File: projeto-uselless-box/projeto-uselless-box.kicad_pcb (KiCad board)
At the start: 2 copper layers, 128 x 94 mm, 13 parts, among them J2 Conn_Para_Fita, J3 Conn_Para_PowerBank, M1 Motor_Servo-Edit, M2 Motor_Servo-Edit, M3 Motor_Servo-Edit, Q1 TIP41, SW1 SW_DPST_x2

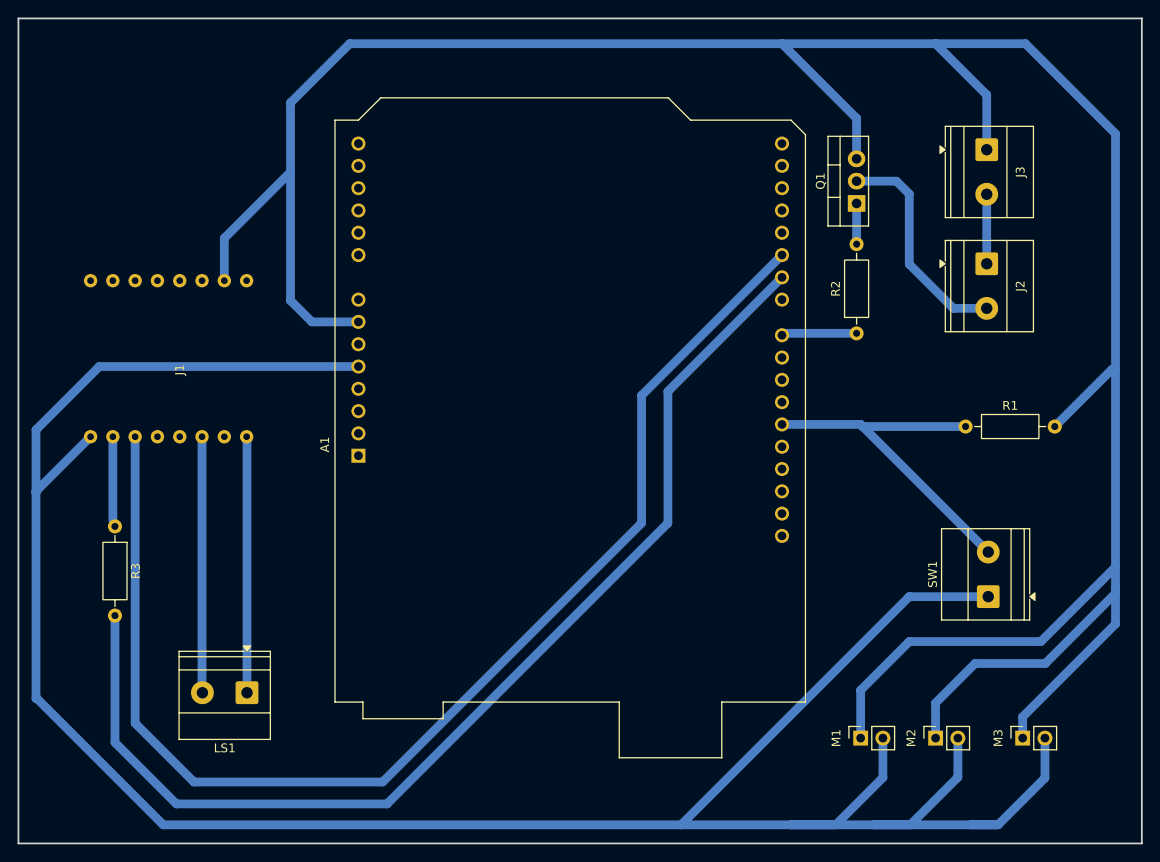
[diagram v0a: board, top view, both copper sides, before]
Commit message: Shorted
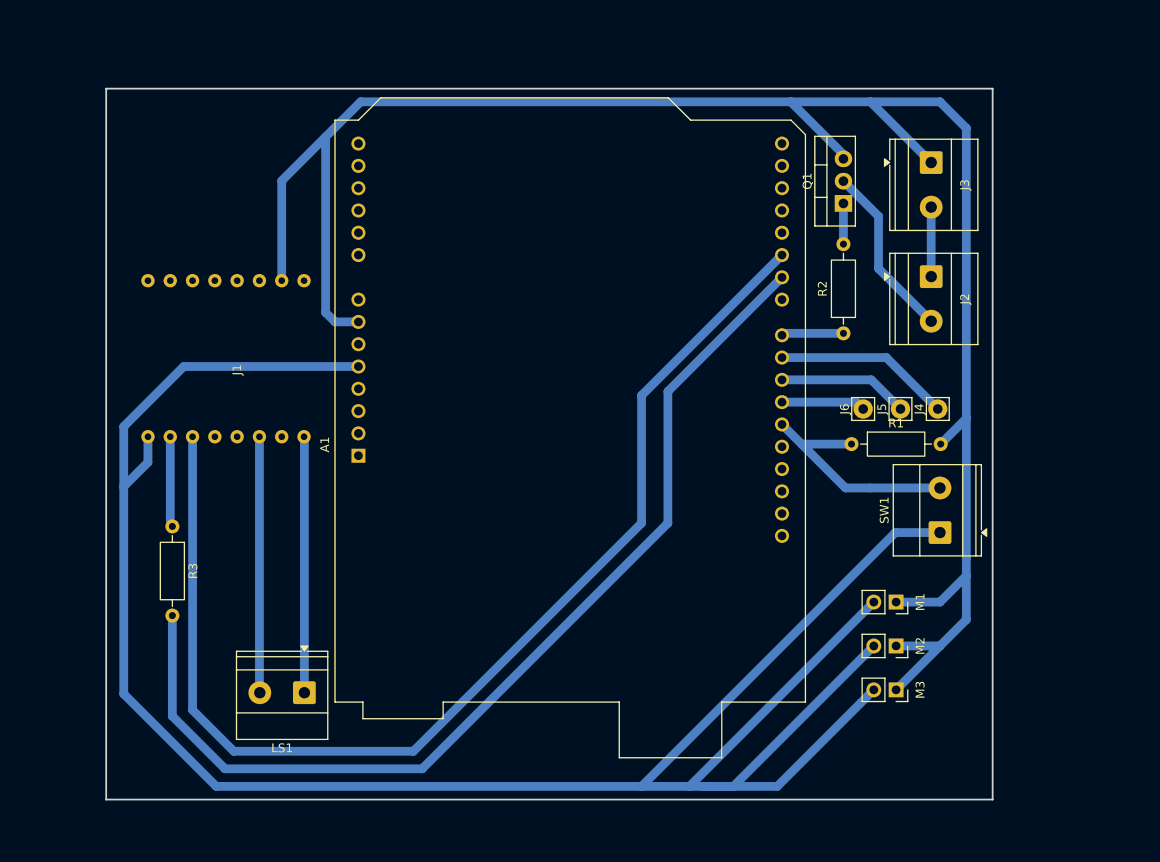
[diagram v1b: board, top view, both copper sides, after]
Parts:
- added J4: Conn_01x01_Pin, Connector_Pin:Pin_D1.1mm_L8.5mm_W2.5mm_FlatFork, F.Cu at (174.8, 97.0)
- added J5: Conn_01x01_Pin, Connector_Pin:Pin_D1.1mm_L8.5mm_W2.5mm_FlatFork, F.Cu at (170.5, 97.0)
- added J6: Conn_01x01_Pin, Connector_Pin:Pin_D1.1mm_L8.5mm_W2.5mm_FlatFork, F.Cu at (166.2, 97.0)
- moved M1 16.0 mm to (170.0, 119.0), turned to -90 degrees
- moved M3 15.4 mm to (170.0, 129.0), turned to -90 degrees
- moved R1 13.2 mm to (164.9, 101.0)
- moved M2 11.4 mm to (170.0, 124.0), turned to -90 degrees
- moved SW1 9.14 mm to (175.0, 111.1)
- moved J1 6.54 mm to (84.8, 92.5)
- moved R3 6.54 mm to (87.5, 110.4)
- moved LS1 6.54 mm to (102.6, 129.3)
- moved J2 6.49 mm to (174.0, 81.9)
- moved J3 6.49 mm to (174.0, 68.9)
- moved Q1 1.50 mm to (164.0, 73.6)
- moved R2 1.50 mm to (164.0, 88.4)
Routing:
- net GND: track 332.3 -> 223.1 mm
- net +5V: track 289.2 -> 263.0 mm
- net D9: track 0.00 -> 20.2 mm
- net D12: track 41.6 -> 26.7 mm
- net D10: track 0.00 -> 14.9 mm
- net D6: track 127.0 -> 115.4 mm
- net D5: track 142.5 -> 132.2 mm
- net D11: track 0.00 -> 9.57 mm
- net Net-(J2-Pin_2): track 25.5 -> 20.1 mm
- net D8: track 8.59 -> 7.09 mm
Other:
- board size 128 x 94 mm -> 101 x 81 mm
